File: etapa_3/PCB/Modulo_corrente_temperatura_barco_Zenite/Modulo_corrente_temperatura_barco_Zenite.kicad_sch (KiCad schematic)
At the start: 46 parts, among them J1 RJ45_Shielded, J2 Conn_01x03, U2 LM7805, U3 TLV9004IDR, U4 MCP2515-xSO, U5 MCP2551-I-SN, Y1 16MHz

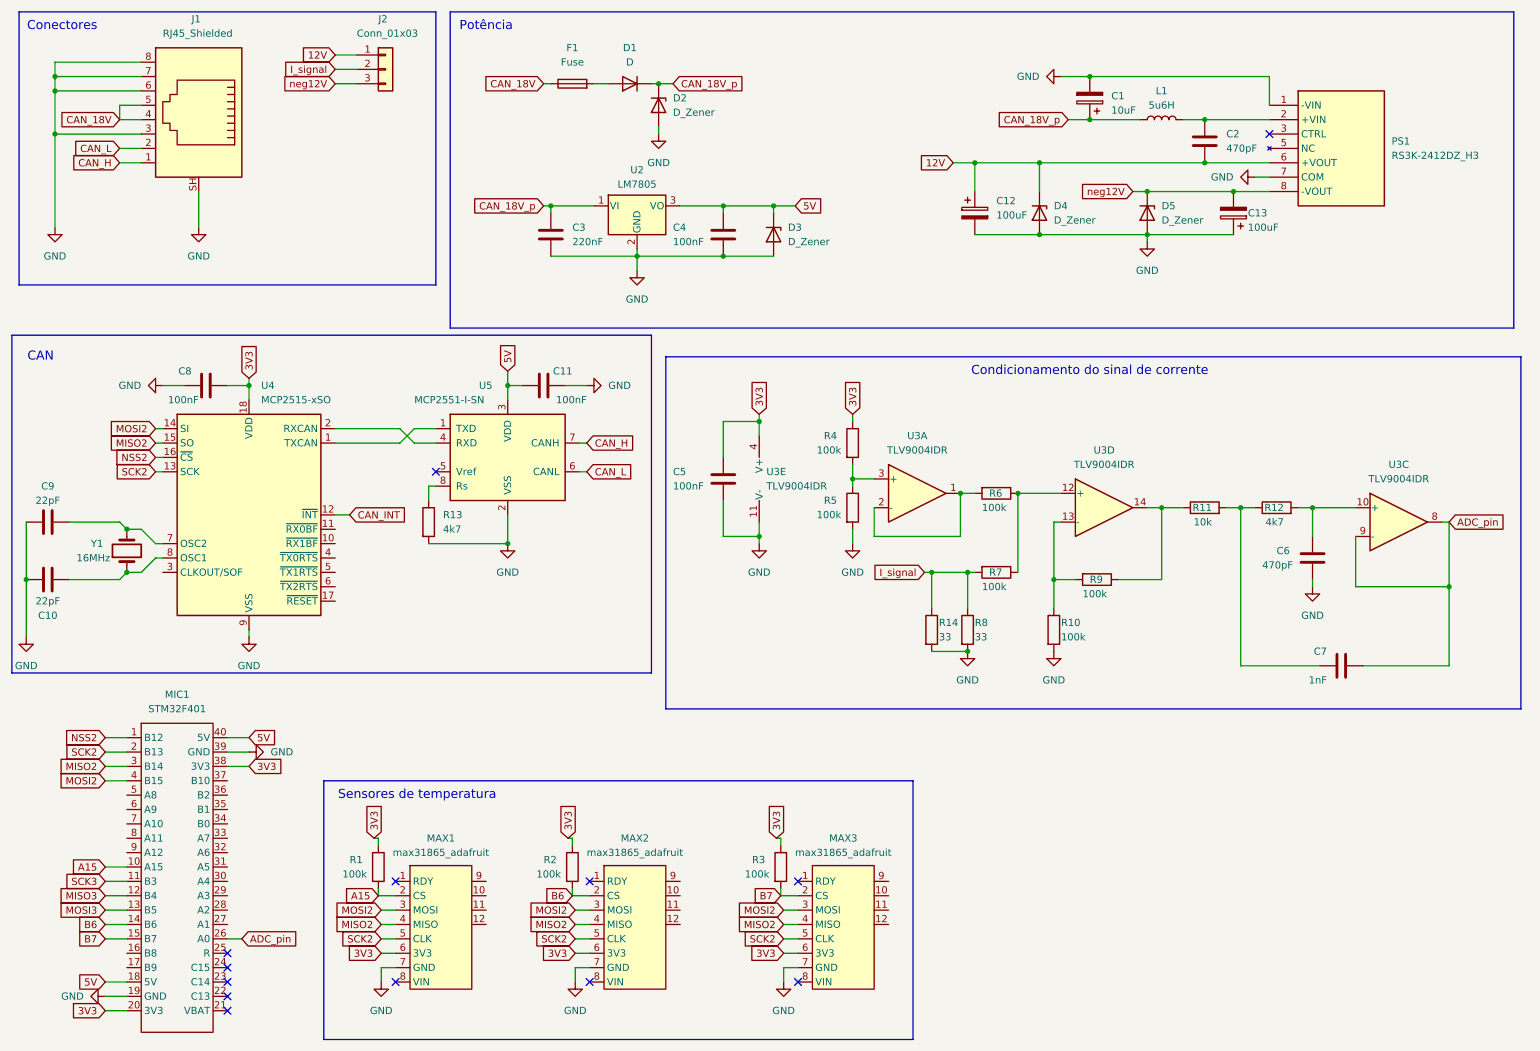
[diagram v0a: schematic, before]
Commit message: update readme.rst
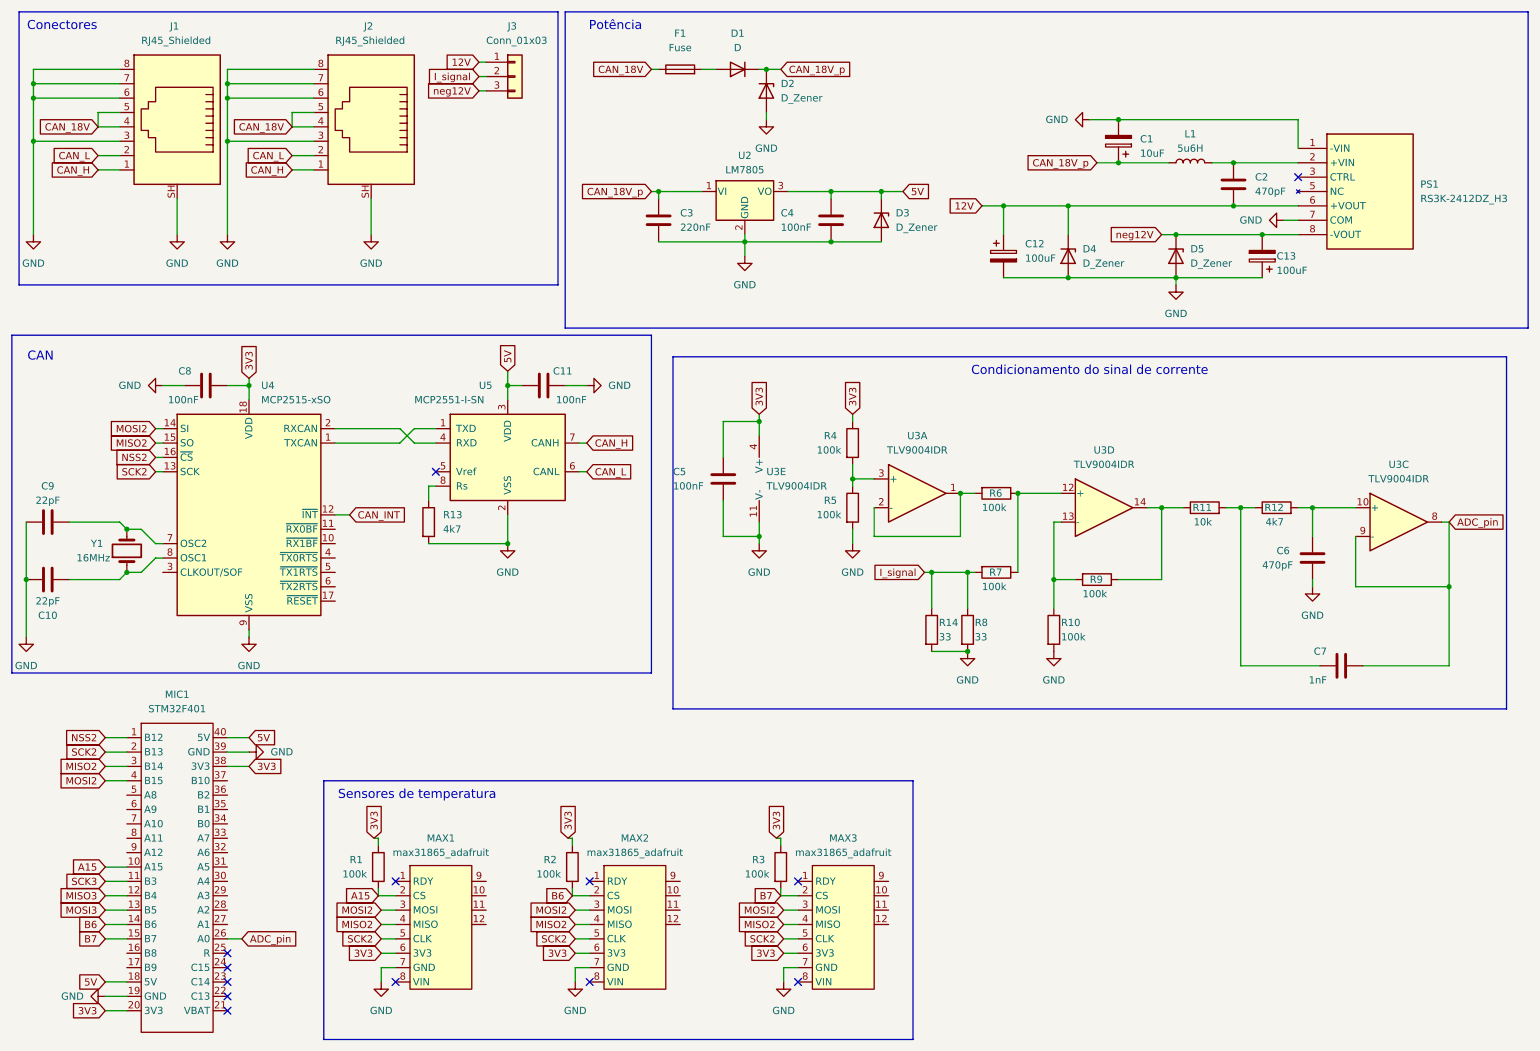
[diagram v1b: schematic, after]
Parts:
- added J2: RJ45_Shielded, symbol Connector:RJ45_Shielded
- renumbered J2 to J3
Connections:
- net CAN_18V: now also J2.4, J2.5
- net CAN_H: now also J2.1
- net CAN_L: now also J2.2
- net GND: now also J2.3, J2.6, J2.7, J2.8, J2.SH
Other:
- moved on the sheet: C1, C12, C13, C2, C3, C4, D1, D2, D3, D4, D5, F1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
